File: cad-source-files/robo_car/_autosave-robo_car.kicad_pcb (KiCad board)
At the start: 2 copper layers, 100 x 100 mm, 94 parts, among them J1 Conn_01x06_MountingPin, J16 Conn_01x02_MountingPin, J2 ftdi_conn, J3 Conn_01x06_MountingPin, J4 Barrel_Jack, J5 Conn_01x04, J6 Conn_01x06_MountingPin, J7 Conn_01x02_MountingPin, J8 Conn_01x02_MountingPin, SW1 SW_Push, SW2 SW_Push, U1 XL1509, U2 AMS1117-3.3, U3 ESP32-WROOM-32U, U4 MOTOR_DRIVER-LV8548MC-AH

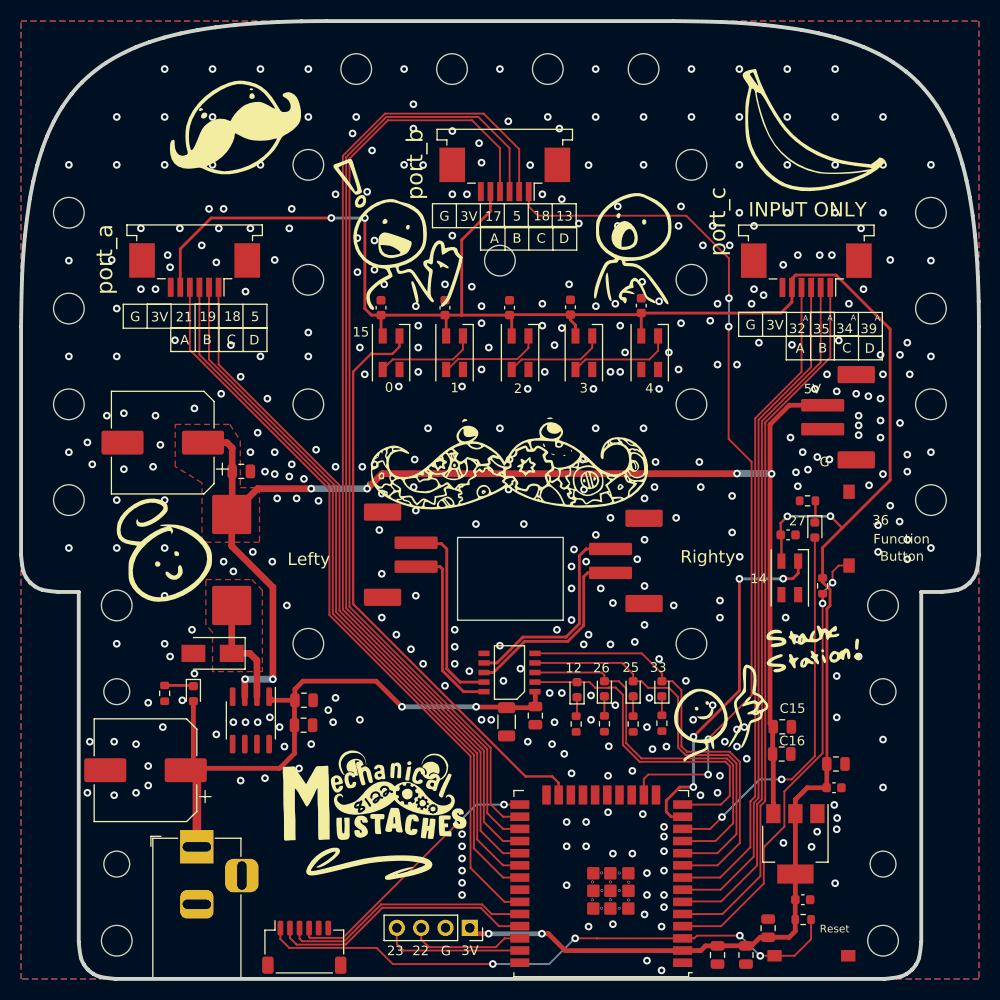
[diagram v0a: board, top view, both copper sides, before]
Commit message: Revert "3rd try lets go"
This reverts commit 3f093a060dbc0dc4159fd1f3f57facfb81c75c62.
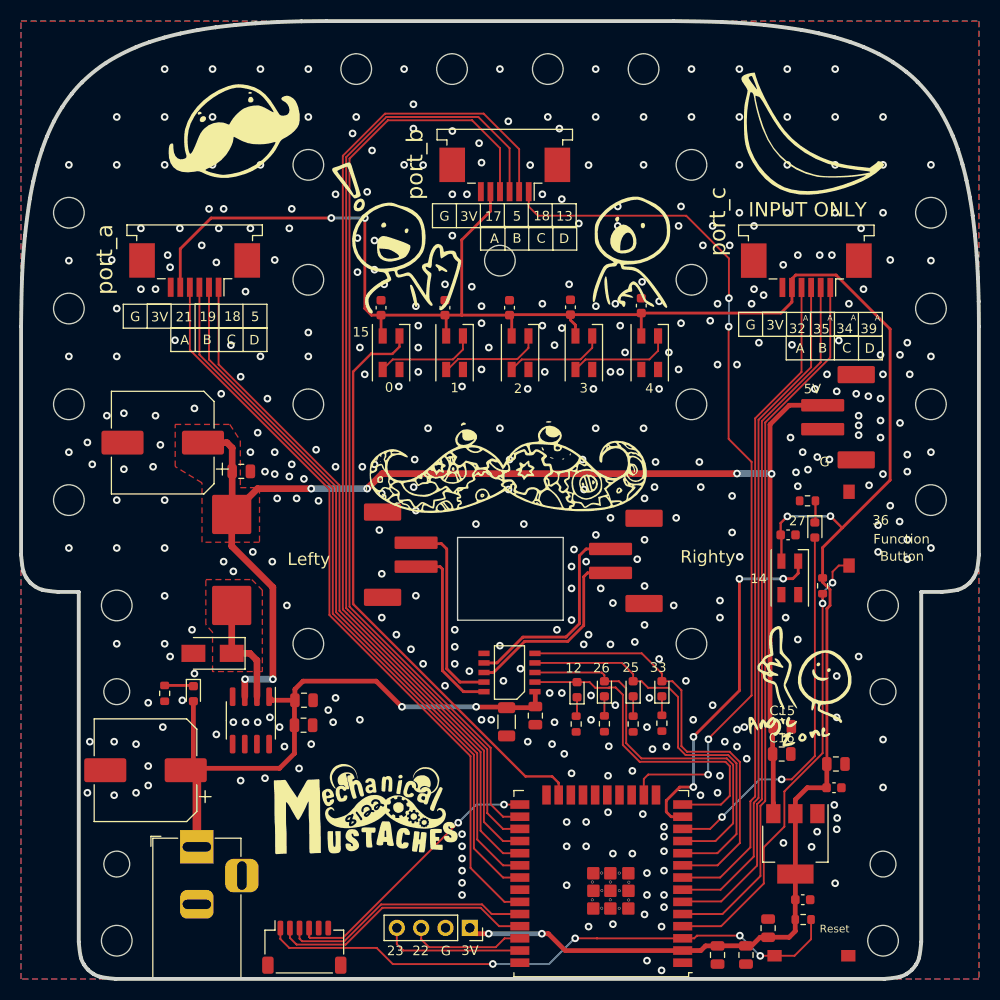
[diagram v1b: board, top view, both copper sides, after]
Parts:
- removed the G*** at (150.3, 98.4)
- removed the G*** at (150.6, 104.0)
- removed the G*** at (150.9, 100.9)
- removed the G*** at (152.4, 102.3)
- added G***: LOGO, Drawing:mustache, F.Cu at (150.8, 101.3)
- moved G*** 1.69 mm to (135.9, 132.9)
